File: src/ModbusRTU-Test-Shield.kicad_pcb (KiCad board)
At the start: 2 copper layers, 68.6 x 53.3 mm, 46 parts, among them J1 SP-140520-08-001, J2 SP-140520-10-001, J3 SP-140520-08-001, J4 SP-140520-06-001, J5 5430438, J6 54601-906WPLF, SW1 BUTTON1, SW2 BUTTON2, SW3 RESET, SW4 OS202011MS2QN1, U1 RS-485 XCVR, U2 RS-232 XCVR

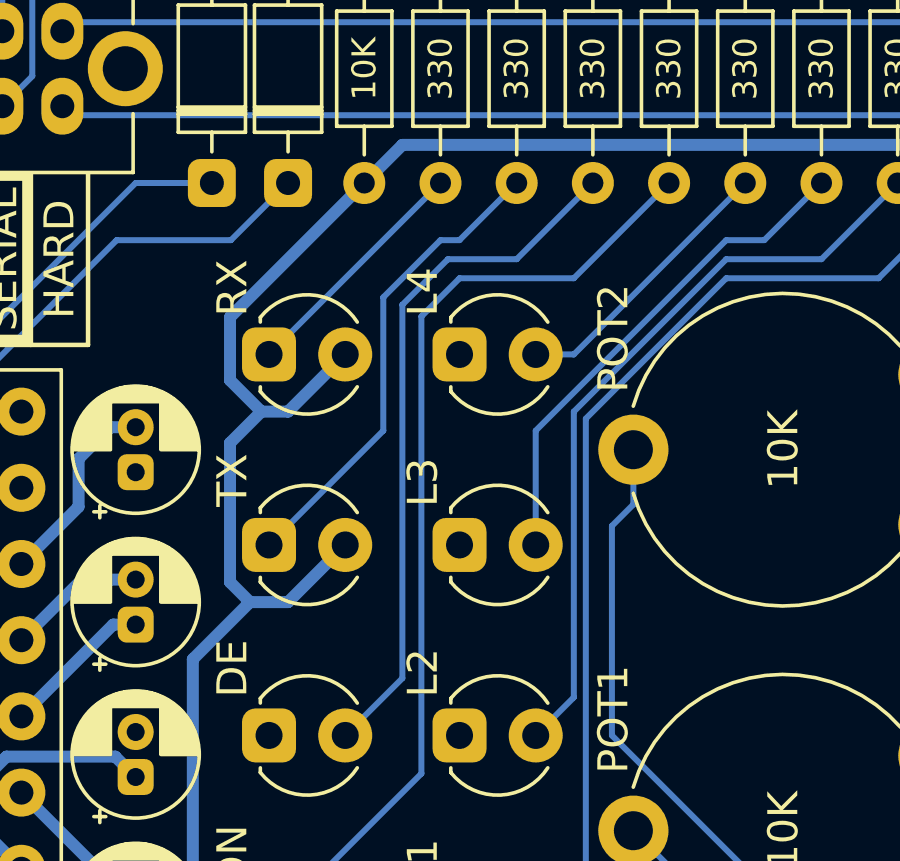
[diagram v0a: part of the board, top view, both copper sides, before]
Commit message: Updated the source files.
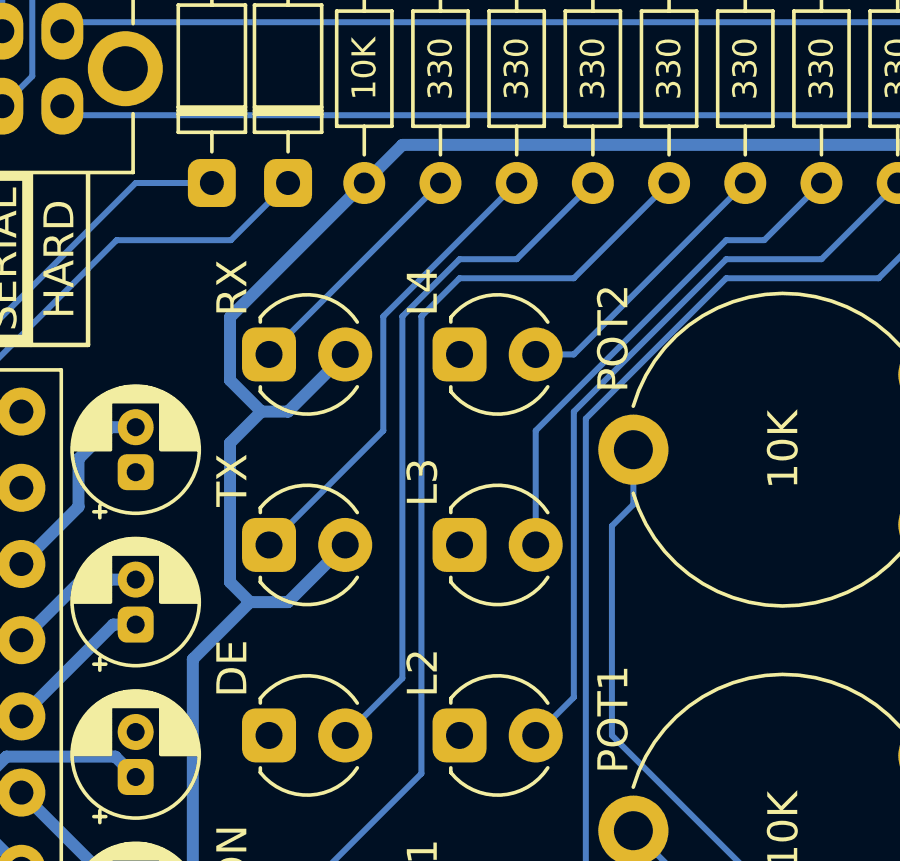
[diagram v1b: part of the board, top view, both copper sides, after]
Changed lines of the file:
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@@
     (grid_origin 105.41 134.62)
     (pcbplotparams
-      (layerselection 0x0000100_7ffffffe)
-      (plot_on_all_layers_selection 0x0021220_00000000)
+      (layerselection 0x00010f0_ffffffff)
+      (plot_on_all_layers_selection 0x0000000_00000000)
       (disableapertmacros false)
       (usegerberextensions false)
@@
       (dashed_line_gap_ratio 3.000000)
       (svgprecision 6)
-      (plotframeref true)
+      (plotframeref false)
       (viasonmask false)
       (mode 1)
-      (useauxorigin false)
+      (useauxorigin true)
       (hpglpennumber 1)
       (hpglpenspeed 20)
@@
       (sketchpadsonfab false)
       (subtractmaskfromsilk true)
-      (outputformat 4)
+      (outputformat 1)
       (mirror false)
       (drillshape 0)
       (scaleselection 1)
-      (outputdirectory "../")
+      (outputdirectory "../gerbers/")
     )
   )
@@
   (segment (start 145.415 102.235) (end 146.685 100.965) (width 0.2) (layer "B.Cu") (net 21))
   (segment (start 145.415 117.475) (end 145.415 102.235) (width 0.2) (layer "B.Cu") (net 21))
-  (segment (start 150.495 100.965) (end 153.67 97.79) (width 0.2) (layer "B.Cu") (net 21))
-  (segment (start 140.335 122.555) (end 145.415 117.475) (width 0.2) (layer "B.Cu") (net 21))
   (segment (start 146.685 100.965) (end 150.495 100.965) (width 0.2) (layer "B.Cu") (net 21))
+  (segment (start 140.335 122.555) (end 145.415 117.475) (width 0.2) (layer "B.Cu") (net 21))
+  (segment (start 150.495 100.965) (end 153.67 97.79) (width 0.2) (layer "B.Cu") (net 21))
   (segment (start 135.14 112.51) (end 135.89 112.51) (width 0.4) (layer "B.Cu") (net 22))
   (segment (start 132.08 115.57) (end 135.14 112.51) (width 0.4) (layer "B.Cu") (net 22))
@@
   (segment (start 133.985 108.585) (end 133.985 106.986472) (width 0.4) (layer "B.Cu") (net 27))
   (segment (start 135.041472 105.93) (end 135.89 105.93) (width 0.4) (layer "B.Cu") (net 27))
-  (segment (start 142.875 116.205) (end 144.78 114.3) (width 0.2) (layer "B.Cu") (net 32))
-  (segment (start 144.78 114.3) (end 144.78 101.848186) (width 0.2) (layer "B.Cu") (net 32))
+  (segment (start 146.685 100.33) (end 148.59 100.33) (width 0.2) (layer "B.Cu") (net 32))
+  (segment (start 144.78 114.3) (end 144.78 102.235) (width 0.2) (layer "B.Cu") (net 32))
+  (segment (start 144.78 102.235) (end 146.685 100.33) (width 0.2) (layer "B.Cu") (net 32))
   (segment (start 148.59 100.33) (end 151.13 97.79) (width 0.2) (layer "B.Cu") (net 32))
-  (segment (start 146.298186 100.33) (end 148.59 100.33) (width 0.2) (layer "B.Cu") (net 32))
-  (segment (start 144.78 101.848186) (end 146.298186 100.33) (width 0.2) (layer "B.Cu") (net 32))
+  (segment (start 142.875 116.205) (end 144.78 114.3) (width 0.2) (layer "B.Cu") (net 32))
   (segment (start 143.51 90.17) (end 146.05 90.17) (width 0.2) (layer "B.Cu") (net 33))
   (segment (start 131.445 95.23) (end 132.445 94.23) (width 0.2) (layer "B.Cu") (net 33))
@@
   (segment (start 140.97 90.17) (end 143.51 90.17) (width 0.2) (layer "B.Cu") (net 33))
   (segment (start 132.445 94.23) (end 132.445 91.5) (width 0.2) (layer "B.Cu") (net 33))
-  (segment (start 144.145 106.045) (end 144.145 101.6) (width 0.2) (layer "B.Cu") (net 34))
-  (segment (start 144.145 101.6) (end 146.05 99.695) (width 0.2) (layer "B.Cu") (net 34))
-  (segment (start 146.685 99.695) (end 148.59 97.79) (width 0.2) (layer "B.Cu") (net 34))
-  (segment (start 146.05 99.695) (end 146.685 99.695) (width 0.2) (layer "B.Cu") (net 34))
   (segment (start 140.335 109.855) (end 144.145 106.045) (width 0.2) (layer "B.Cu") (net 34))
+  (segment (start 144.145 106.045) (end 144.145 102.235) (width 0.2) (layer "B.Cu") (net 34))
+  (segment (start 144.145 102.235) (end 148.59 97.79) (width 0.2) (layer "B.Cu") (net 34))
   (segment (start 168.91 88.265) (end 168.91 83.82) (width 0.2) (layer "B.Cu") (net 35))
   (segment (start 133.445 95.23) (end 133.745 95.53) (width 0.2) (layer "B.Cu") (net 35))
